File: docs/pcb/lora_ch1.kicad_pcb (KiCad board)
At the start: 2 copper layers, 69 x 34 mm, 22 parts, among them J2 TYPE-C-31-M-12, J3 JST_2mm_LiPo, U1 ESP32-C3_SUPERMINI_TH, U2 TP4056-42-ESOP8, U3 DRV2605LDGS, U4 AP2112K-3.3

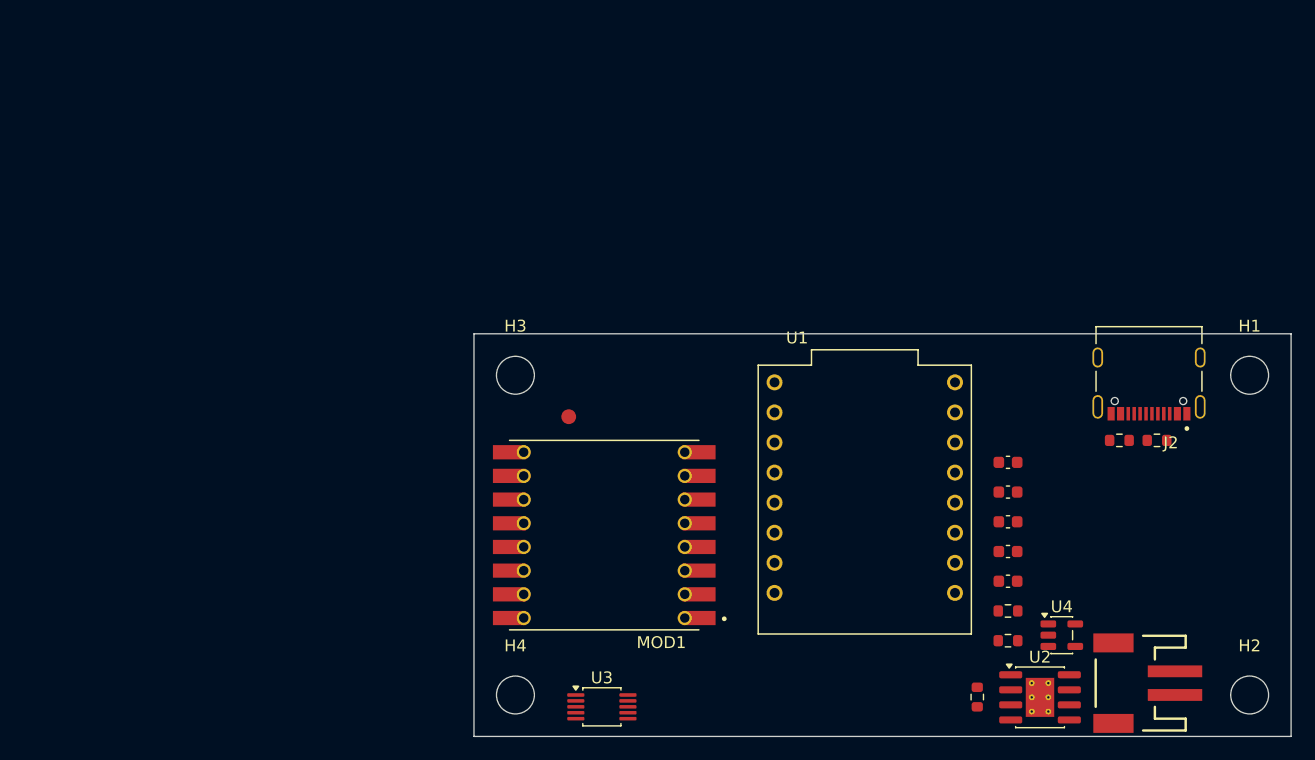
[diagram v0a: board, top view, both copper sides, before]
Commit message: PCB schematic finished.
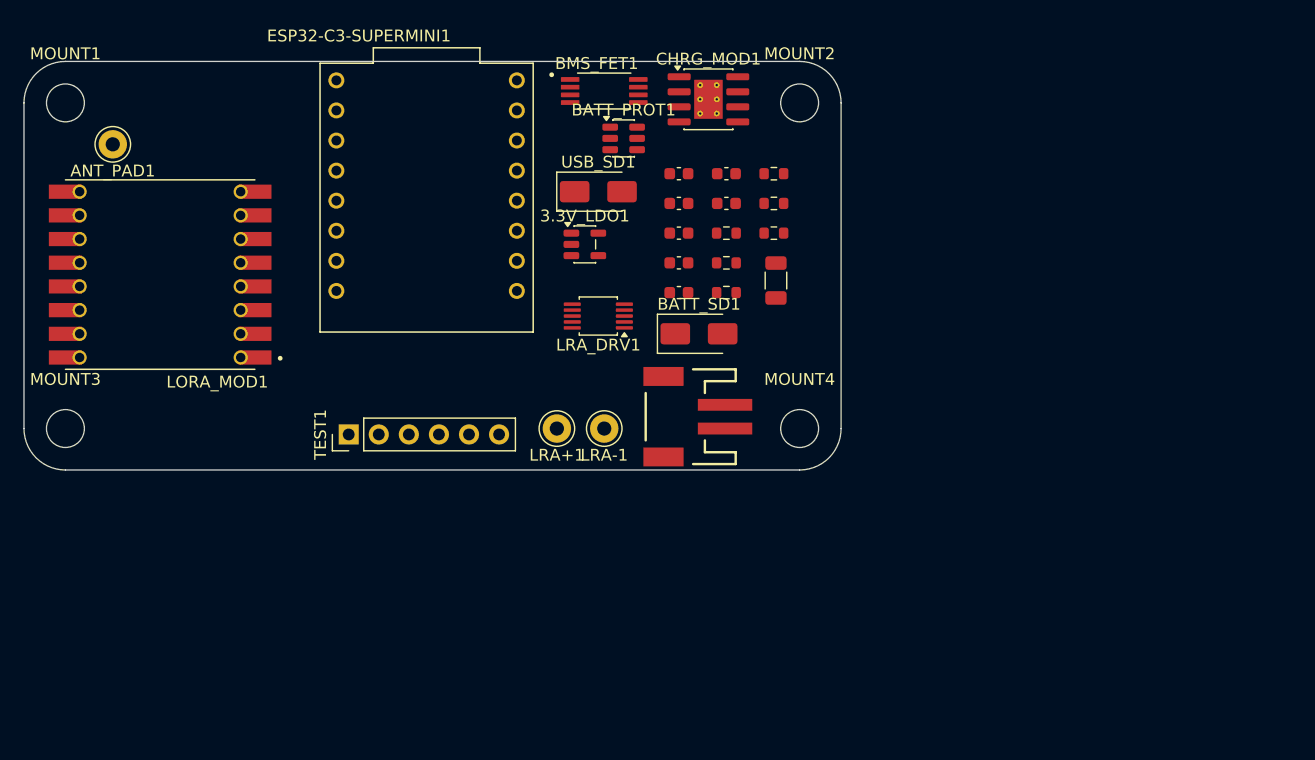
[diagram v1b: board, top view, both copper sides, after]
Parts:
- removed H1, H2, H3, H4: MountingHole_M3, MountingHole:MountingHole_3.2mm_M3
- removed J2: TYPE-C-31-M-12, TYPE-C-31-M-12:HRO_TYPE-C-31-M-12
- removed J3: JST_2mm_LiPo, PCM_SparkFun-Connector:JST_1x02_P2.0mm_Horizontal_SMD
- removed MOD1: RFM98W-433S2, RFM98W-433S2:XCVR_RFM98W-433S2
- removed R3: 5.1k, PCM_SparkFun-Resistor:R_0603_1608Metric
- removed TP1: 1.25mm, PCM_SparkFun-Connector:TestPoint-1.25mm
- removed U1: ESP32-C3_SUPERMINI_TH, ESP32-C3_SUPERMINI_TH:MODULE_ESP32-C3_SUPERMINI_TH
- removed U2: TP4056-42-ESOP8, Package_SO:SOIC-8-1EP_3.9x4.9mm_P1.27mm_EP2.41x3.3mm_ThermalVias
- removed U3: DRV2605LDGS, Package_SO:VSSOP-10_3x3mm_P0.5mm
- removed U4: AP2112K-3.3, Package_TO_SOT_SMD:SOT-23-5
- added 3.3V_LDO1: XC6220B331MR, Package_TO_SOT_SMD:SOT-23-5, F.Cu at (122.4, 75.5)
- added ANT_PAD1: PINHD_1x1_Male, Connector_Pin:Pin_D1.0mm_L10.0mm_LooseFit, F.Cu at (82.5, 67.0)
- added BATT_CON1: JST_2mm_LiPo, PCM_SparkFun-Connector:JST_1x02_P2.0mm_Horizontal_SMD, F.Cu at (130.5, 90.0)
- added BATT_PROT1: DW01A, Package_TO_SOT_SMD:SOT-23-6, F.Cu at (125.6, 66.5)
- added BATT_SD1: SS14, Diode_SMD:D_SMA, F.Cu at (132.0, 83.0)
- added BMS_FET1: FS8205A, FS8205A:SOP65P640X120-8N, F.Cu at (124.0, 62.5)
- added C6: 100uF, PCM_SparkFun-Capacitor:C_1206_3216Metric, F.Cu at (138.5, 78.5)
- added C7: 100nF, PCM_SparkFun-Capacitor:C_0603_1608Metric, F.Cu at (134.3, 69.5)
- added C8: 1.0uF, PCM_SparkFun-Capacitor:C_0603_1608Metric, F.Cu at (134.3, 72.0)
- added CHRG_MOD1: TP4056-42-ESOP8, Package_SO:SOIC-8-1EP_3.9x4.9mm_P1.27mm_EP2.41x3.3mm_ThermalVias, F.Cu at (132.8, 63.2)
- added ESP32-C3-SUPERMINI1: ESP32-C3_SUPERMINI_TH, ESP32-C3_SUPERMINI_TH:MODULE_ESP32-C3_SUPERMINI_TH, F.Cu at (109.0, 71.5)
- added LORA_MOD1: RFM98W-433S2, RFM98W-433S2:XCVR_RFM98W-433S2, F.Cu at (86.5, 78.0)
- added LRA+1: PINHD_1x1_Male, Connector_Pin:Pin_D1.0mm_L10.0mm_LooseFit, F.Cu at (120.0, 91.0)
- added LRA-1: PINHD_1x1_Male, Connector_Pin:Pin_D1.0mm_L10.0mm_LooseFit, F.Cu at (124.0, 91.0)
- added LRA_DRV1: DRV2605LDGS, Package_SO:VSSOP-10_3x3mm_P0.5mm, F.Cu at (123.5, 81.5)
- added MOUNT1: MountingHole_M3, MountingHole:MountingHole_3.2mm_M3, F.Cu at (78.5, 63.5)
- added MOUNT2: MountingHole_M3, MountingHole:MountingHole_3.2mm_M3, F.Cu at (140.5, 63.5)
- added MOUNT3: MountingHole_M3, MountingHole:MountingHole_3.2mm_M3, F.Cu at (78.5, 91.0)
- added MOUNT4: MountingHole_M3, MountingHole:MountingHole_3.2mm_M3, F.Cu at (140.5, 91.0)
- added R6: 100, PCM_SparkFun-Resistor:R_0603_1608Metric, F.Cu at (138.3, 72.0)
- added R7: 1k, PCM_SparkFun-Resistor:R_0603_1608Metric, F.Cu at (138.3, 74.5)
- added TEST1: PINHD_1x6_Male, Connector_PinHeader_2.54mm:PinHeader_1x06_P2.54mm_Vertical, F.Cu at (102.4, 91.5)
- added USB_SD1: SS14, Diode_SMD:D_SMA, F.Cu at (123.5, 71.0)
- C1, C3, C4: value 0.1uF -> 10uF
- moved R1 44.5 mm to (134.3, 74.5), turned to 0 degrees
- moved R5 44.1 mm to (138.3, 69.5)
- moved C1 37.0 mm to (130.3, 69.5)
- moved C2 37.0 mm to (130.3, 72.0)
- moved C3 37.0 mm to (130.3, 74.5)
- moved C4 37.0 mm to (130.3, 77.0)
- moved C5 37.0 mm to (130.3, 79.5)
- moved R2 36.4 mm to (134.3, 77.0)
- moved R4 35.9 mm to (134.3, 79.5)
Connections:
- C1 pad 1: Net-(U3-VDD) -> GND
- C1 pad 2: GND -> 3.3V
- C2 pad 1: +3.3V -> GND
- C2 pad 2: GND -> V_IN
- C3 pad 2: Net-(U3-REG) -> V_USB
- C4 pad 1: +3.3V -> VBAT+
- C5 pad 1: 3.3V -> GND
- C5 pad 2: +3.3V -> V_IN
- R1 pad 1: Net-(U2-PROG) -> GND
- R1 pad 2: GND -> Net-(CHRG_MOD1-PROG)
- R2 pad 1: GND -> 3.3V
- R2 pad 2: Net-(J2-CC1) -> LORA_NSS
- R4 pad 1: +3.3V -> SDA
- R4 pad 2: SDA -> 3.3V
- R5 pad 1: SCL -> 3.3V
- R5 pad 2: +3.3V -> SCL
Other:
- board size 69 x 34 mm -> 69 x 34.5 mm
